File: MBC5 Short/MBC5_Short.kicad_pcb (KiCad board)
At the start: 2 copper layers, 51 x 30.7 mm, 1 part, among them J1 GameBoy_GamePak_AGB-002

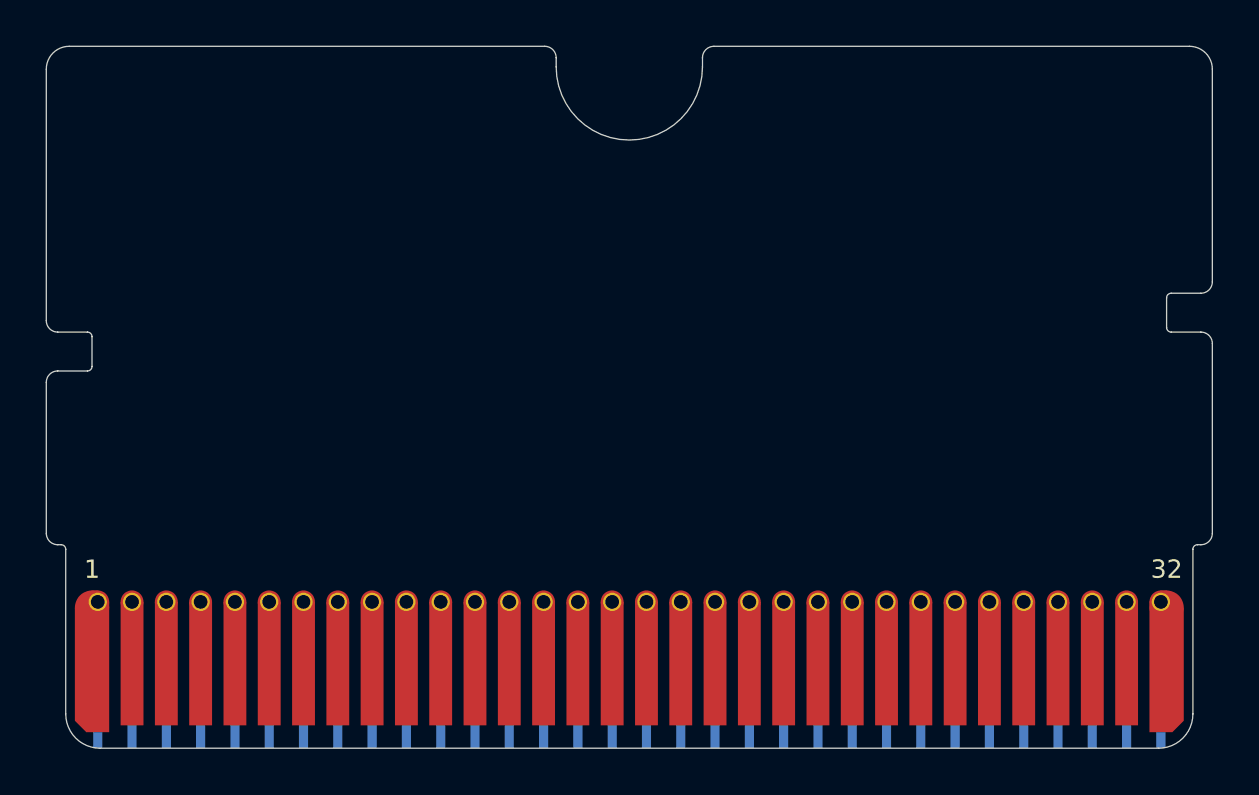
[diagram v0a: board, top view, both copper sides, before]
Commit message: Initialize PCB configuration (blank template)
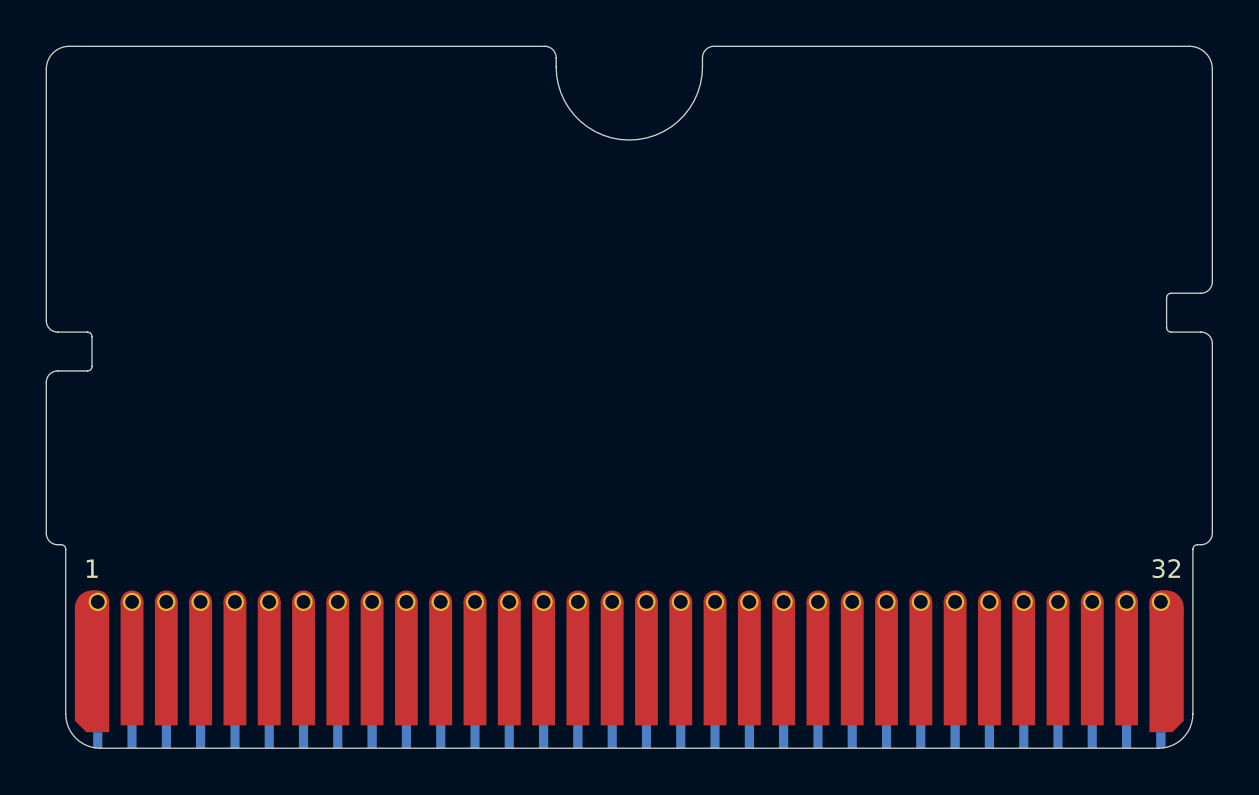
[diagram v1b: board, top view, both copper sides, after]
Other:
- outline, holes or cut-outs redrawn
- net class Default removed
